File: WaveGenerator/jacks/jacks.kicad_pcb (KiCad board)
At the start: 2 copper layers, 41.9 x 16.5 mm, 9 parts, among them J1 Conn_01x06, J2 TRIGGER, J3 TRIG, J4 PWM, J5 PWM, J6 VOUT, J7 VOUT, J8 Conn_01x04, J9 Conn_01x04

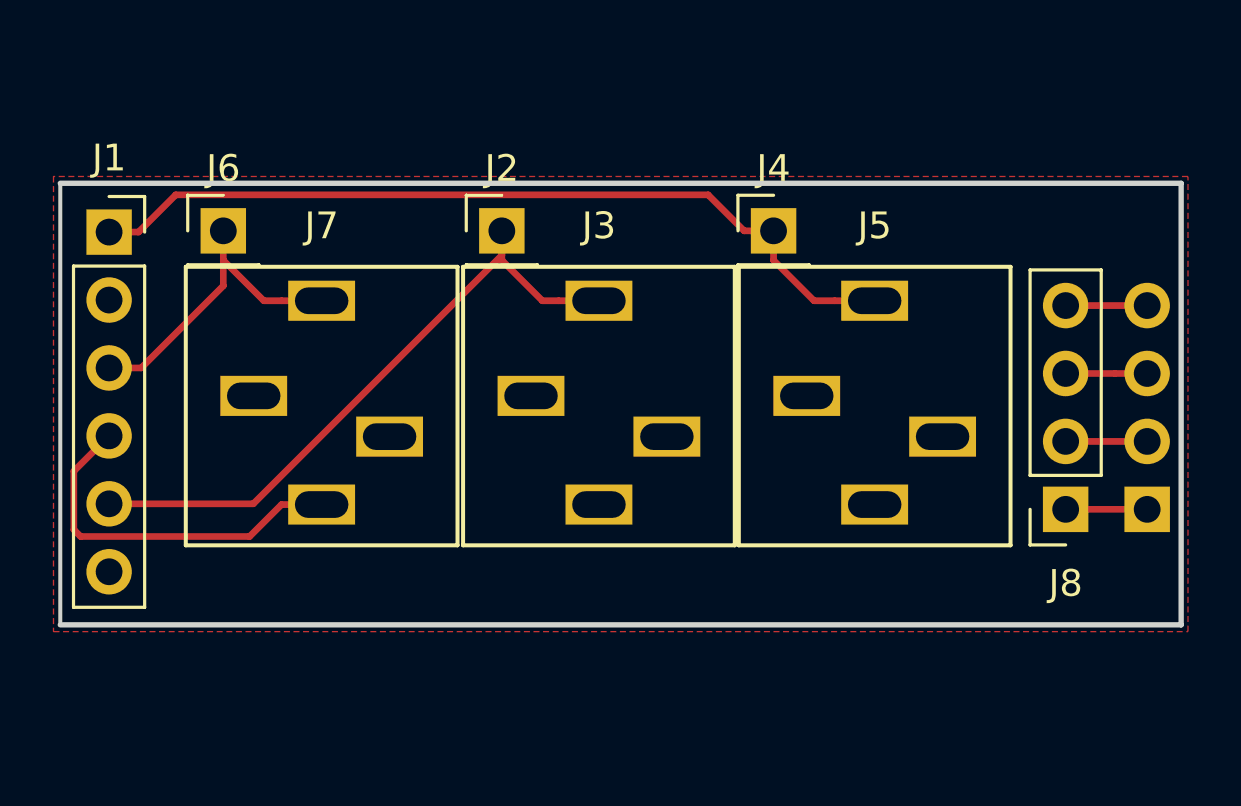
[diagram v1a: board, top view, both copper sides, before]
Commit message: Wave gerber panelized
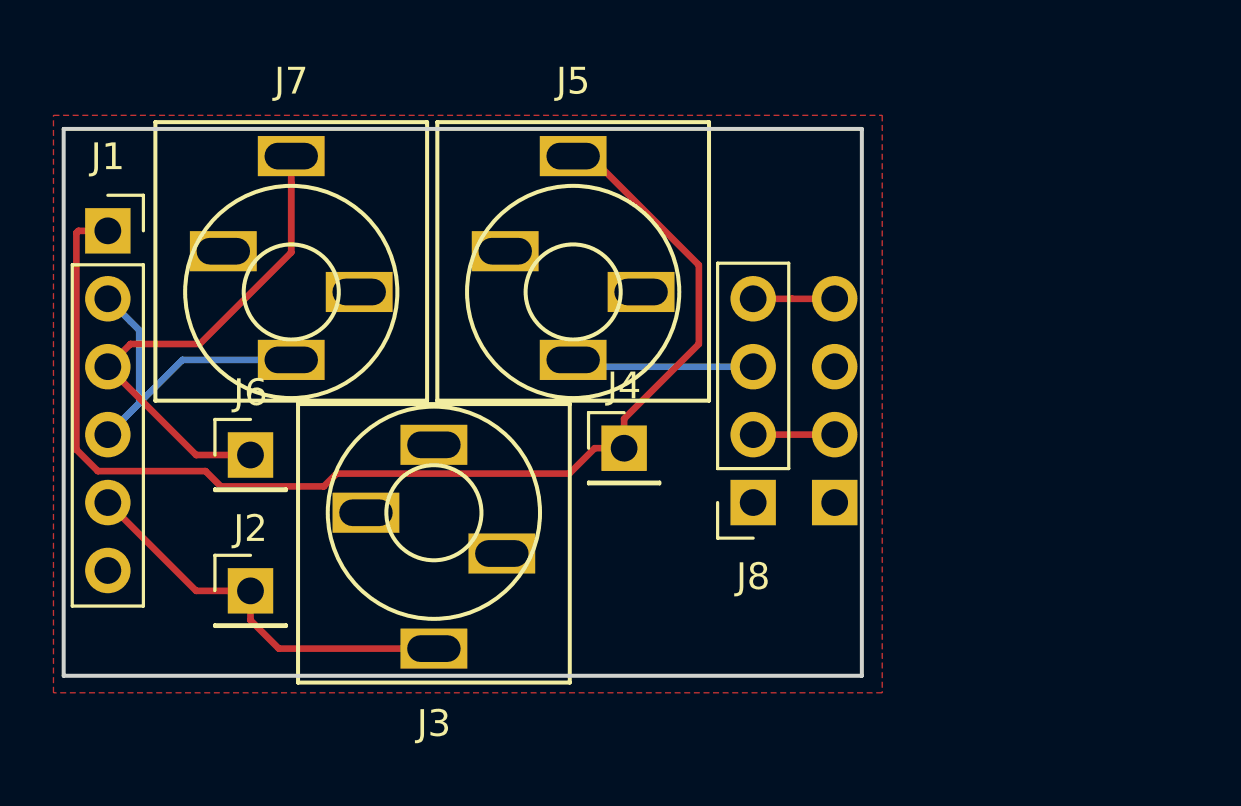
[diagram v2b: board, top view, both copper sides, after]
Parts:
- moved J2 16.4 mm to (82.0, 111.8)
- moved J5 12.5 mm to (94.1, 100.6)
- moved J8 11.7 mm to (100.8, 108.5)
- moved J9 11.7 mm to (103.9, 108.5)
- moved J4 9.86 mm to (96.0, 106.4)
- moved J6 8.44 mm to (82.0, 106.7)
- moved J3 6.80 mm to (88.9, 108.8), turned to 180 degrees
- moved J7 5.53 mm to (83.6, 100.6)
- moved J1 0.07 mm to (76.7, 98.3)
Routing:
- net PWM: track 31.5 -> 45.2 mm
- net TRIGGER: track 24.8 -> 15.1 mm
- net VOUT_: track 11.9 -> 18.9 mm
- net GND: track 20.0 -> 21.0 mm
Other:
- board size 41.9 x 16.5 mm -> 29.8 x 20.4 mm
